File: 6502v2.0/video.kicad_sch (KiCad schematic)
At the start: 15 parts, among them J17 Conn_Coaxial, Q3 NPN, U12 TMS9918A, U16 74LS574, U17 74LS574, U18 74LS574, U19 HM62256BLP, U20 74HC04, Y1 Crystal

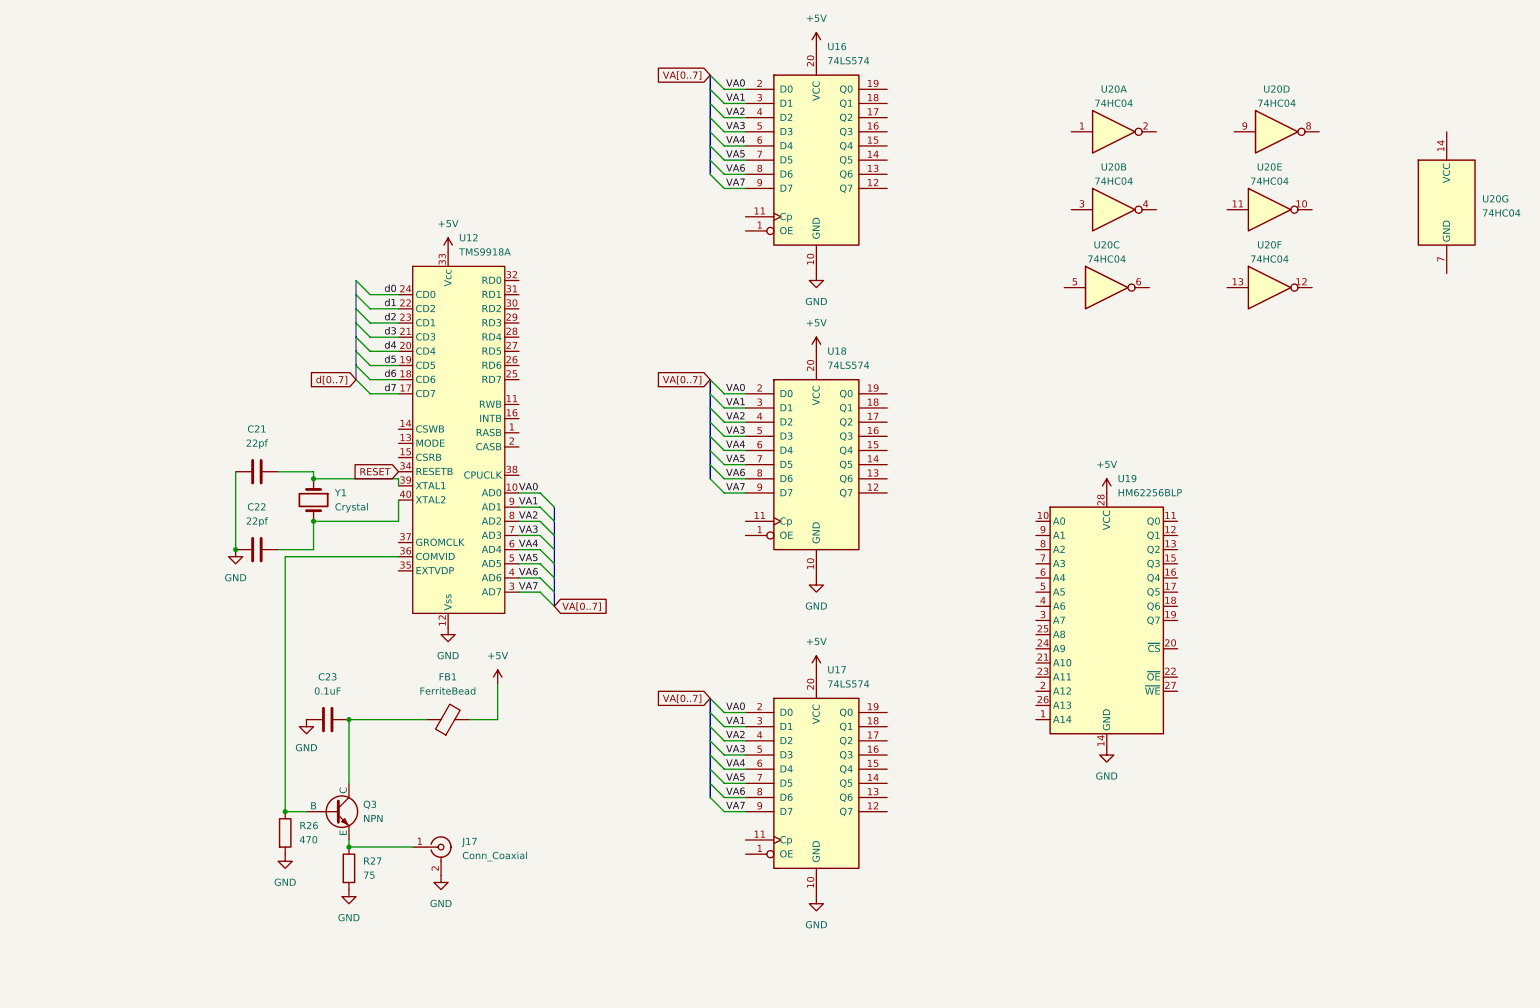
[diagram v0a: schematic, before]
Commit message: worked on video card
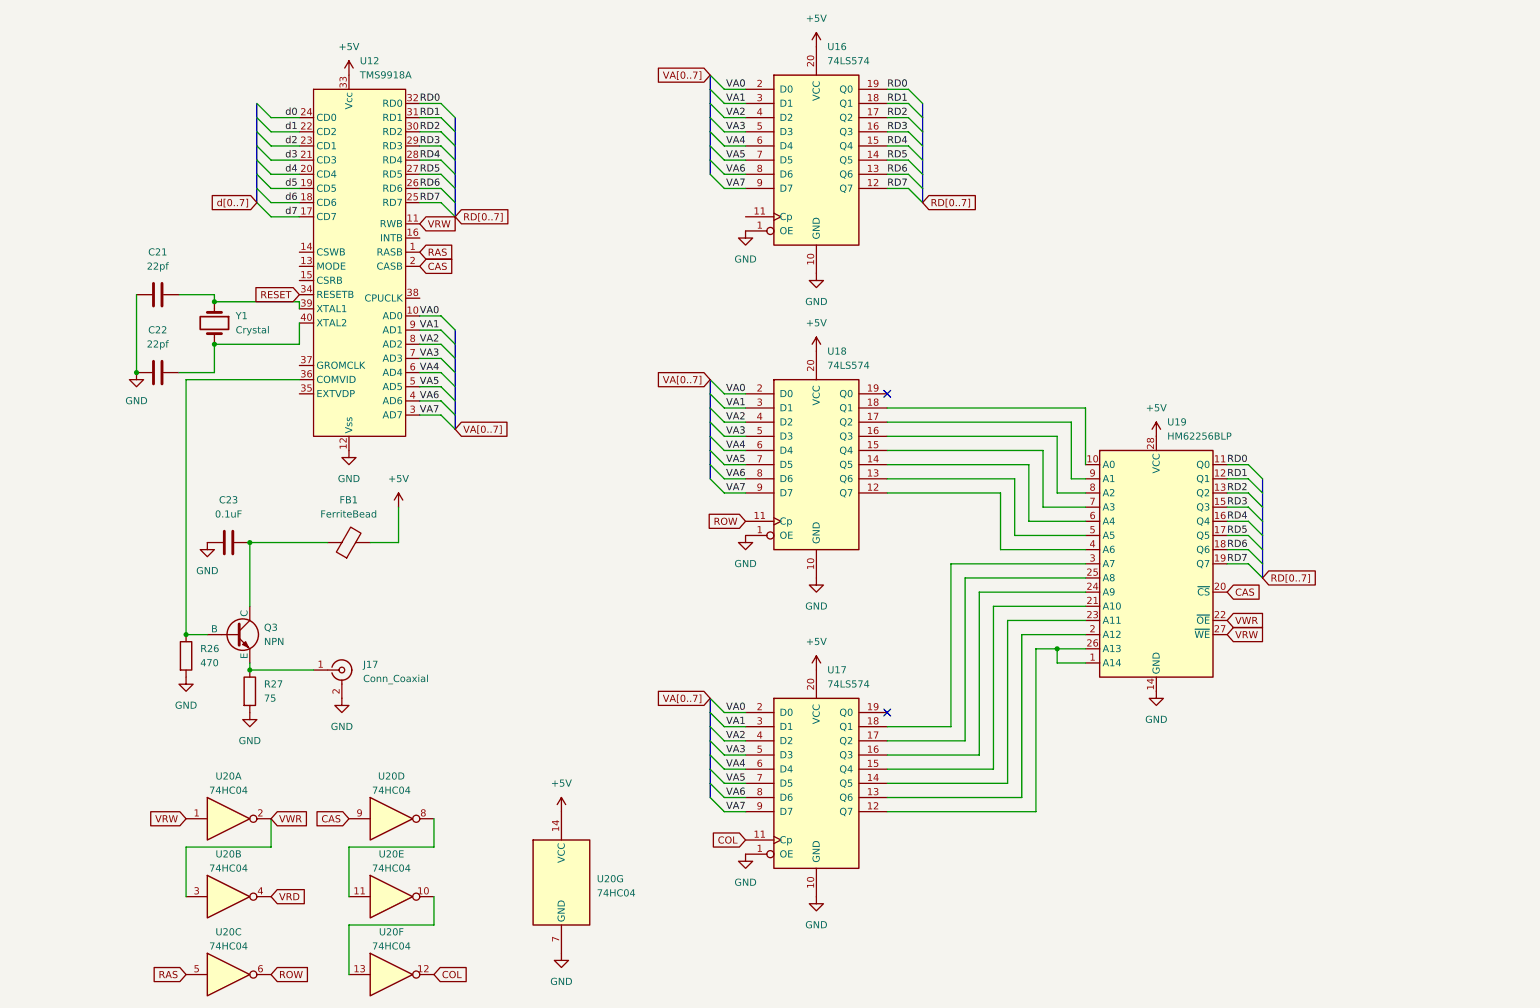
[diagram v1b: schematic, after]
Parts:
- U12: footprint Package_DIP:DIP-40_W15.24mm_Socket -> (none)
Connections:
- net +5V: now also U20.14 (VCC)
- net GND: now also U16.1 (OE), U17.1 (OE), U18.1 (OE), U20.7 (GND)
- net RAS: now reaches U12.1 (RASB)
- net RAS: now also U20.5
- net VRW: now reaches U12.11 (RWB)
- net VRW: now also U19.27 (~{WE}), U20.1
- net CAS: now reaches U12.2 (CASB)
- net CAS: now also U19.20 (~{CS}), U20.9
- net RD7: now reaches U12.25 (RD7)
- net RD7: now also U16.12 (Q7), U19.19 (Q7)
- net RD6: now reaches U12.26 (RD6)
- net RD6: now also U16.13 (Q6), U19.18 (Q6)
- net RD5: now reaches U12.27 (RD5)
- net RD5: now also U16.14 (Q5), U19.17 (Q5)
- net RD4: now reaches U12.28 (RD4)
- net RD4: now also U16.15 (Q4), U19.16 (Q4)
- net RD3: now reaches U12.29 (RD3)
- net RD3: now also U16.16 (Q3), U19.15 (Q3)
- net RD2: now reaches U12.30 (RD2)
- net RD2: now also U16.17 (Q2), U19.13 (Q2)
- net RD1: now reaches U12.31 (RD1)
- net RD1: now also U16.18 (Q1), U19.12 (Q1)
- net RD0: now reaches U12.32 (RD0)
- net RD0: now also U16.19 (Q0), U19.11 (Q0)
- net ROW: now reaches U18.11 (Cp)
- net ROW: now also U20.6
- net at U18.12 (Q7): now also U19.4 (A6)
- net at U18.13 (Q6): now also U19.5 (A5)
- net at U18.14 (Q5): now also U19.6 (A4)
- net at U18.15 (Q4): now also U19.7 (A3)
- net at U18.16 (Q3): now also U19.8 (A2)
- net at U18.17 (Q2): now also U19.9 (A1)
- net at U18.18 (Q1): now also U19.10 (A0)
- net at U19.1 (A14): now also U17.12 (Q7), U19.26 (A13)
- net at U19.2 (A12): now also U17.13 (Q6)
- net at U19.21 (A10): now also U17.15 (Q4)
- net VWR: now reaches U19.22 (~{OE})
- net VWR: now also U20.2, U20.3
- net at U19.23 (A11): now also U17.14 (Q5)
- net at U19.24 (A9): now also U17.16 (Q3)
- net at U19.25 (A8): now also U17.17 (Q2)
- net at U19.3 (A7): now also U17.18 (Q1)
- net COL: now reaches U17.11 (Cp)
- net COL: now also U20.12
- net at U20.8: now also U20.11
- net VRD: now reaches U20.4
- net at U20.13: now also U20.10
- no-connect marks 0 -> 2
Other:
- moved on the sheet: C21, C22, C23, FB1, J17, Q3, R26, R27, U19, U20A, U20B, U20C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

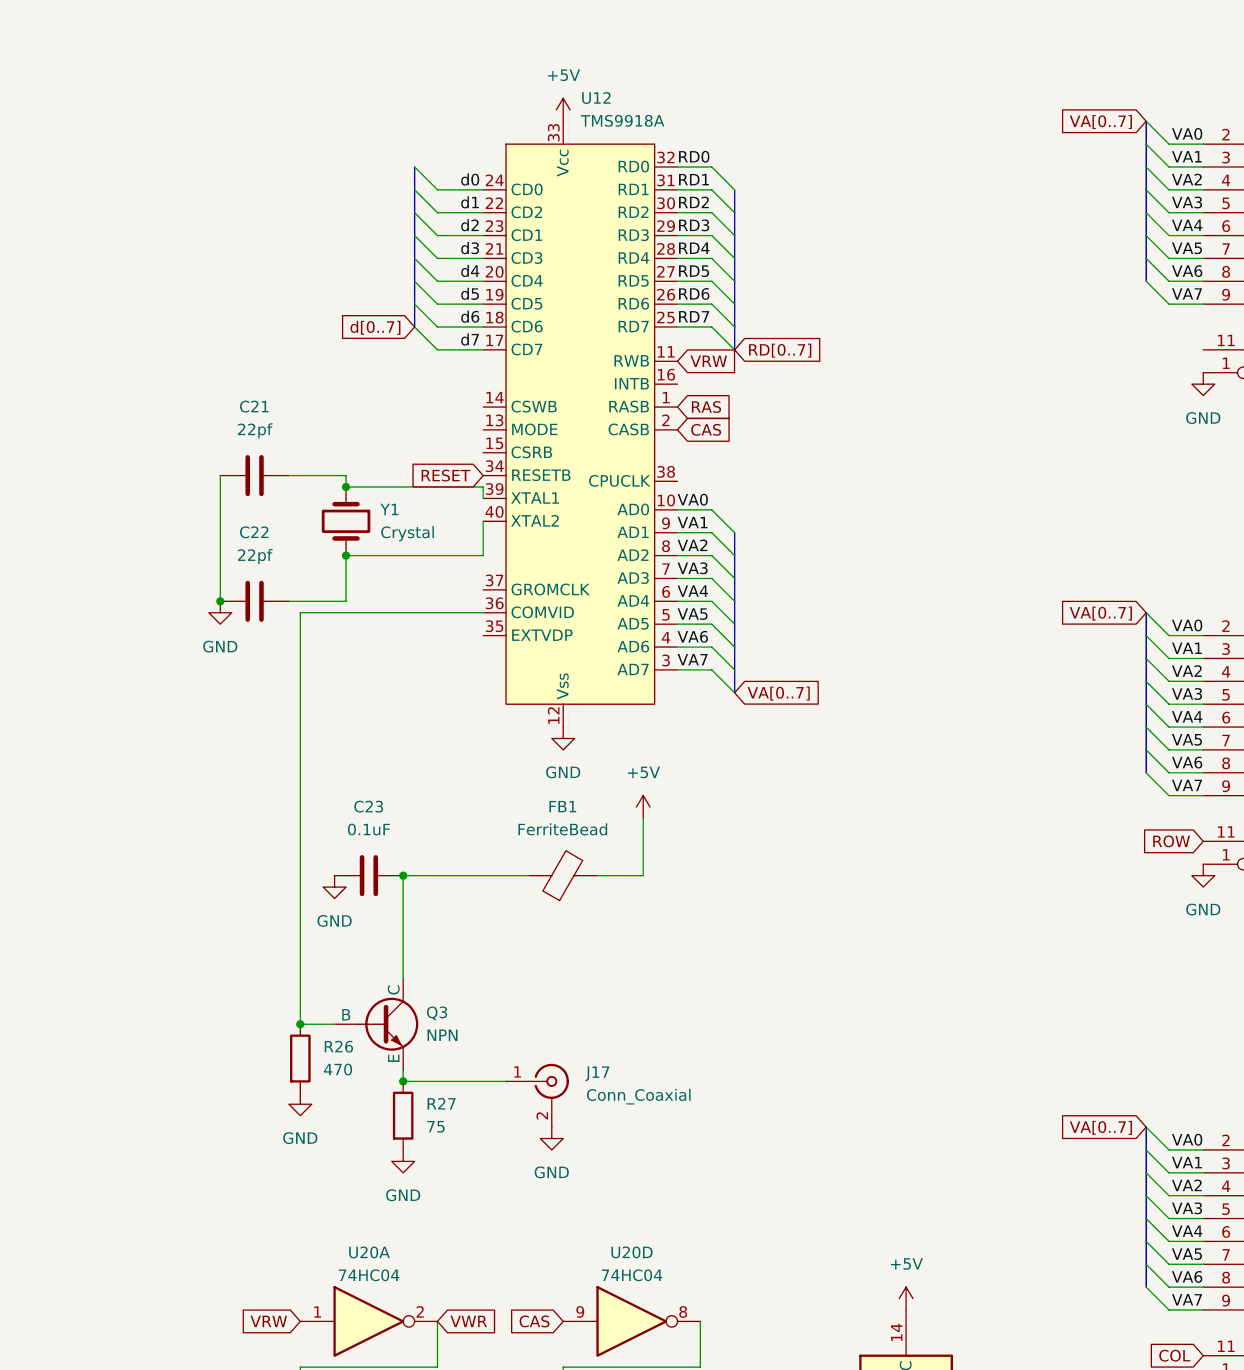
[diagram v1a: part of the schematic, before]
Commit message: changes
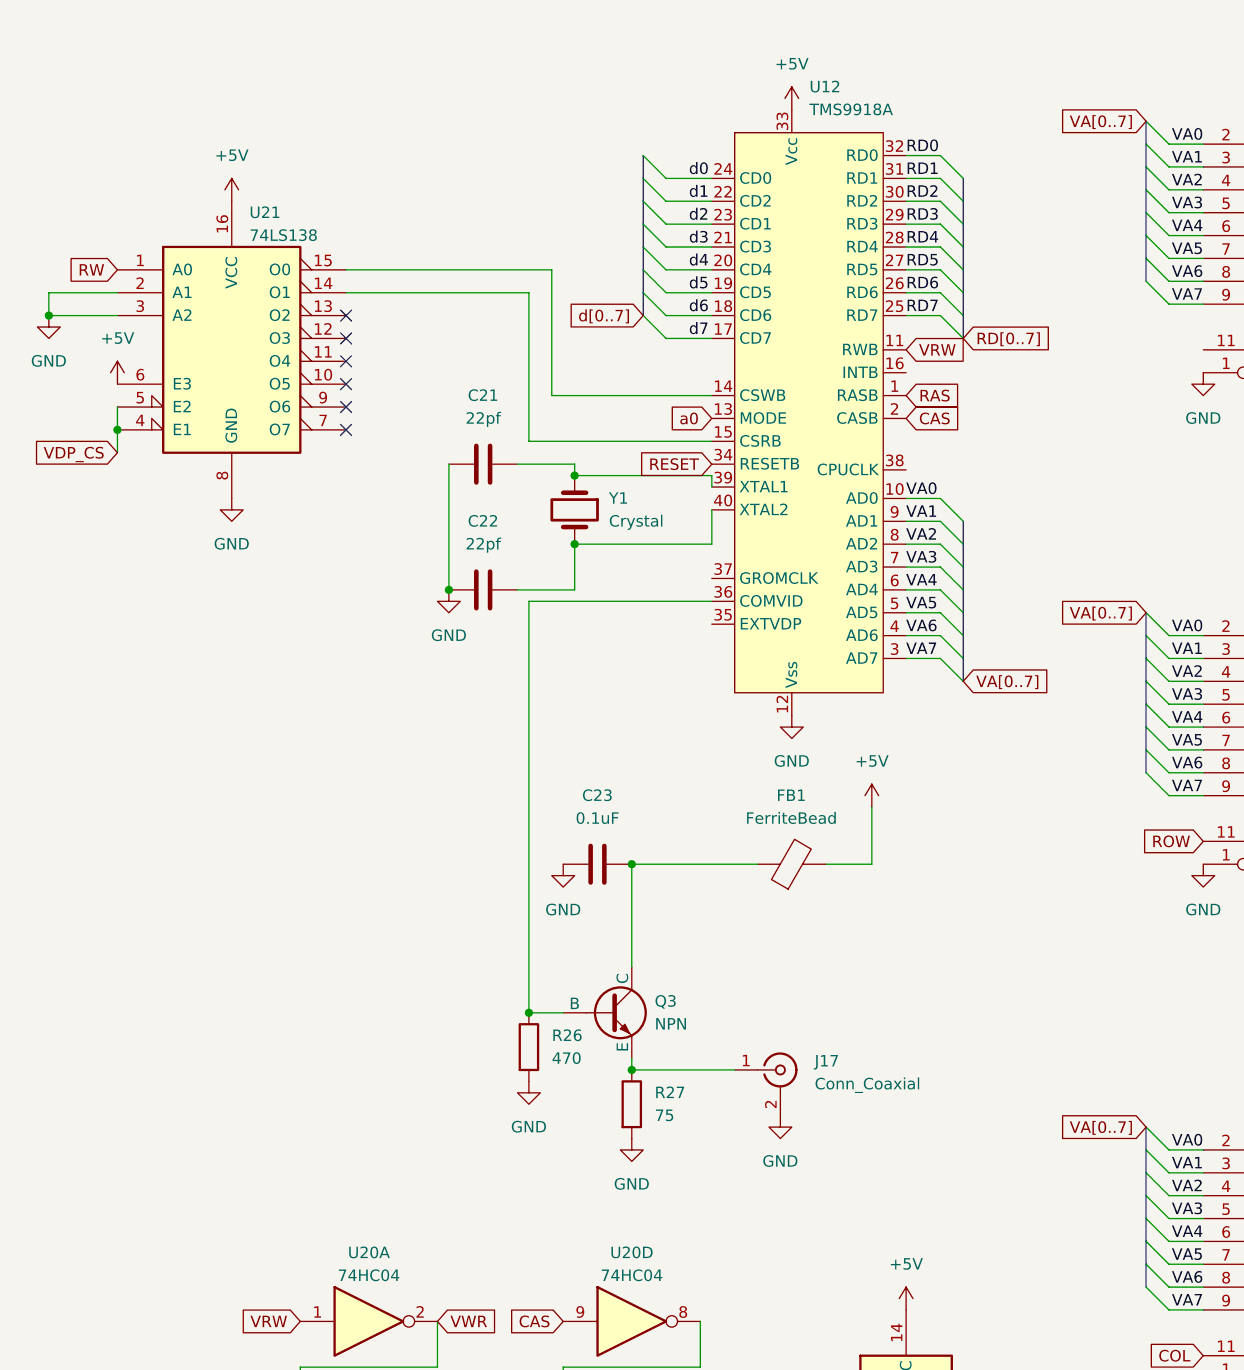
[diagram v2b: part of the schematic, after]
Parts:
- added U21: 74LS138, symbol 74xx:74LS138
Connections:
- net +5V: now also U21.16 (VCC), U21.6 (E3)
- net GND: now also U21.2 (A1), U21.3 (A2), U21.8 (GND)
- net a0: now reaches U12.13 (MODE)
- net at U12.14 (CSWB): now also U21.15 (O0)
- net at U12.15 (CSRB): now also U21.14 (O1)
- new net RW: U21.1 (A0)
- new net VDP_CS: U21.4 (E1), U21.5 (E2)
- no-connect marks 2 -> 8
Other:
- moved on the sheet: C21, C22, C23, FB1, J17, Q3, R26, R27, U12, Y1
